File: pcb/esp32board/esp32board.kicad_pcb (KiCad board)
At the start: 2 copper layers, 122.2 x 54.6 mm, 89 parts, among them J1 1Wire, J10 NTC5, J11 FuelLevel, J12 12V In, J13 Oil Pressure, J14 Engine, J15 Flywheel, J16 Relays, J5 CAN, J6 NTC1, J7 NTC2, J8 NTC3, J9 NTC4, Q1 BS170F, Q2 BS170F, U1 ESP32-C3-Waveshare, U2 AMS1117-5.0, U3 TJA1050, U4 ADS1115IDGS, U5 ADS1115IDGS, U6 ADS1115IDGS, U7 LM393

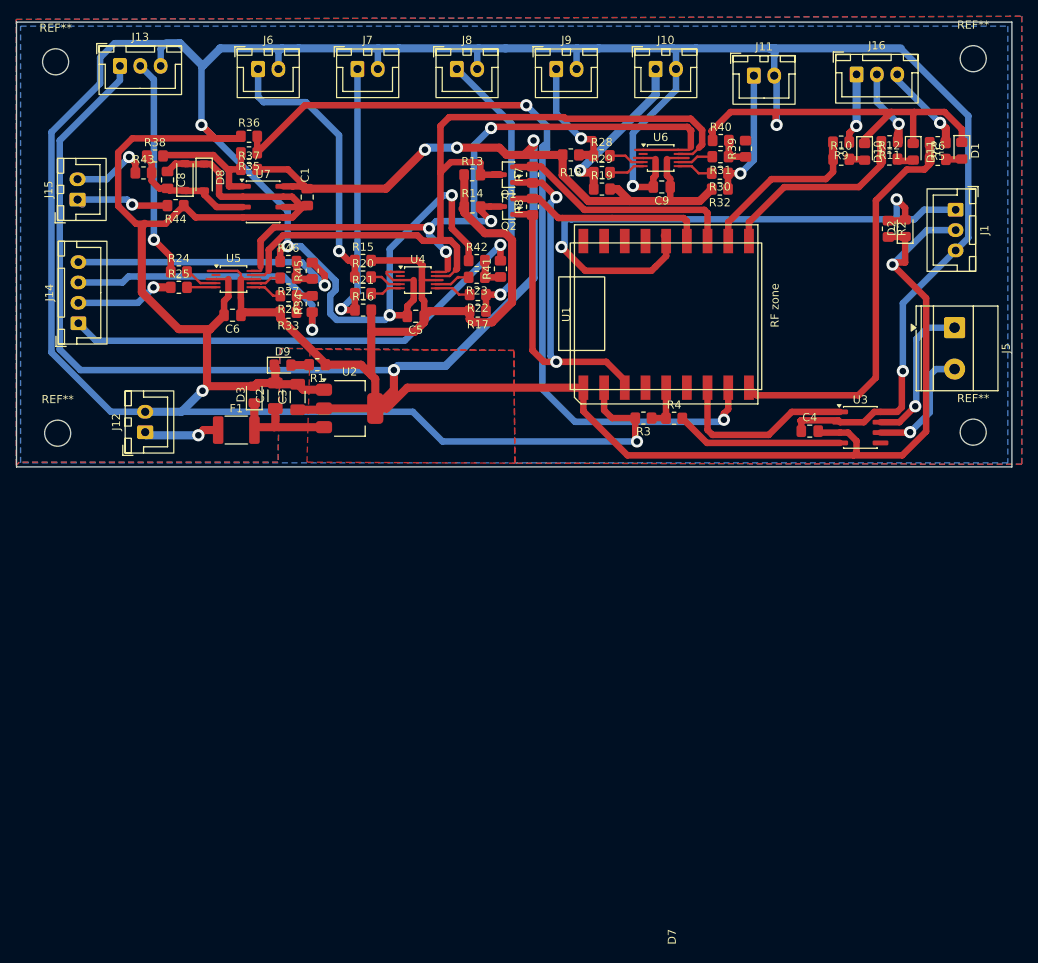
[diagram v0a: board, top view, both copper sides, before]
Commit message: Fixed some hardware problems, new board
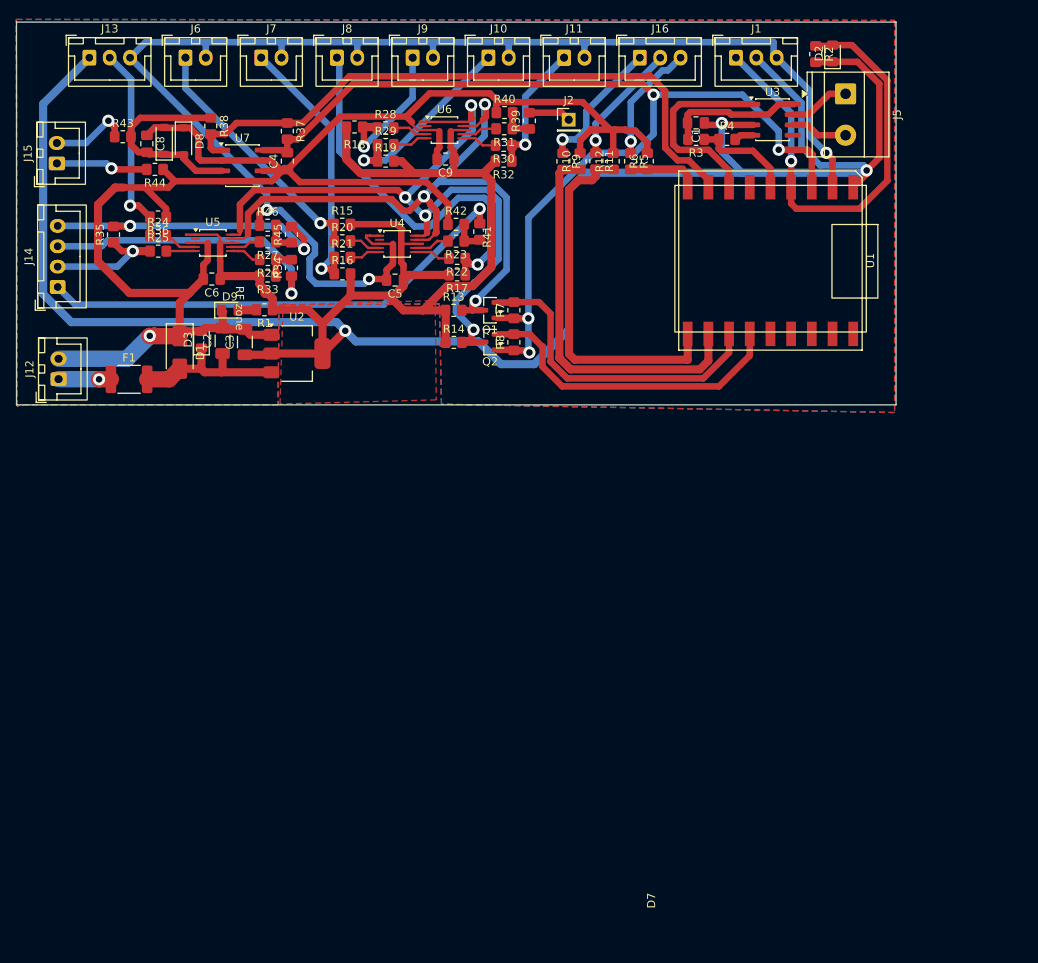
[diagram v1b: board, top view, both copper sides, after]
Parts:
- removed D10, D11: LED, LED_SMD:LED_0805_2012Metric_Pad1.15x1.40mm_HandSolder
- removed REF** (x4): MountingHole_3.2mm_M3, MountingHole:MountingHole_3.2mm_M3
- added J2: V2_spare, Connector_PinHeader_2.54mm:PinHeader_1x01_P2.54mm_Vertical, F.Cu at (139.1, 121.4)
- D1: value LED -> SMAJ16CA; footprint LED_SMD:LED_0805_2012Metric_Pad1.15x1.40mm_HandSolder -> Diode_SMD:D_SMA
- Q1, Q2: value BS170F -> BSS138
- R35: value 2K2 -> 1K
- R36: value 3K3 -> 22K
- R42: value 4K7 -> 3K3
- moved D1 99.2 mm to (91.3, 150.0)
- moved C4 72.2 mm to (104.5, 126.5), turned to 90 degrees
- moved C1 48.6 mm to (154.7, 121.8), turned to 180 degrees
- moved U1 41.6 mm to (174.0, 129.5), turned to -90 degrees
- moved U3 39.3 mm to (164.1, 121.4)
- moved R5 37.8 mm to (146.7, 126.5), turned to -90 degrees
- moved R11 36.1 mm to (142.4, 126.5), turned to -90 degrees
- moved R6 35.7 mm to (148.7, 126.5), turned to 90 degrees
- moved R4 34.8 mm to (158.5, 123.8)
- moved R3 34.8 mm to (154.7, 123.8)
- moved R9 34.2 mm to (138.4, 126.5), turned to -90 degrees
- moved R12 33.9 mm to (144.5, 126.5), turned to 90 degrees
- moved J1 32.8 mm to (159.6, 113.8), turned to 0 degrees
- moved R10 32.1 mm to (140.5, 126.5), turned to 90 degrees
- moved J5 31.7 mm to (173.1, 118.2)
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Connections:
- C2 pad 1: Net-(D3-K) -> Net-(D1-A2)
- C4 pad 2: 5V -> 3v3
- D1 pad 2: Net-(D1-A) -> Net-(D1-A2)
- D3 pad 1: Net-(D3-K) -> Net-(D1-A2)
- F1 pad 2: Net-(D3-K) -> Net-(D1-A2)
- R10 pad 2: Net-(D10-A) -> GND
- R12 pad 2: Net-(D11-A) -> GND
- R35 pad 1: FLYWHEEL -> Coolant
- R35 pad 2: Net-(R35-Pad2) -> Engine Batt+
- R36 pad 2: FLYWHEEL -> OilPressure
- R37 pad 1: Net-(R35-Pad2) -> FLYWHEEL
- R37 pad 2: 5V -> 3v3
- R38 pad 2: Net-(R35-Pad2) -> FLYWHEEL
- R6 pad 2: Net-(D1-A) -> GND
- U1 pad 14: 1-Wire -> unconnected-(U1-GP10-Pad14)
- U1 pad 4: unconnected-(U1-GP0-Pad4) -> 1-Wire
- U2 pad 3: Net-(D3-K) -> Net-(D1-A2)
- U7 pad 1: Net-(R35-Pad2) -> FLYWHEEL
- U7 pad 8: 5V -> 3v3
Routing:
- net GND: track 619.2 -> 408.6 mm, vias 9 -> 4
- net 3v3: track 58.9 -> 129.8 mm, vias 2 -> 4
- net 5V: track 435.0 -> 366.4 mm, vias 5 -> 3
- net STOP: track 49.7 -> 8.83 mm
- net START: track 23.8 -> 50.4 mm
- net FLYWHEEL: track 102.8 -> 77.6 mm, vias 2 -> 0
- net GLOW: track 24.3 -> 45.2 mm
- net Net-(D1-A2): track 0.00 -> 20.6 mm
- net 1-Wire: track 77.1 -> 57.4 mm, vias 2 -> 1
- net Net-(U3-RXD): track 20.6 -> 2.45 mm
- net Net-(R35-Pad2): track 16.1 -> 0.00 mm
- net SDA: track 99.3 -> 83.8 mm, vias 0 -> 3
- net SCL3: track 24.5 -> 39.3 mm
- net Net-(D3-K): track 14.4 -> 0.00 mm
- net NTC3: track 34.8 -> 47.7 mm
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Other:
- board size 122.2 x 54.6 mm -> 108 x 47 mm
- board text added: "${REFERENCE}"
